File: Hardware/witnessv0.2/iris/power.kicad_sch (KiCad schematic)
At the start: 28 parts, among them Q1 SQA403EJ, Q2 SQA403EJ, U2 ME6118A33PG, U6 TPS63070

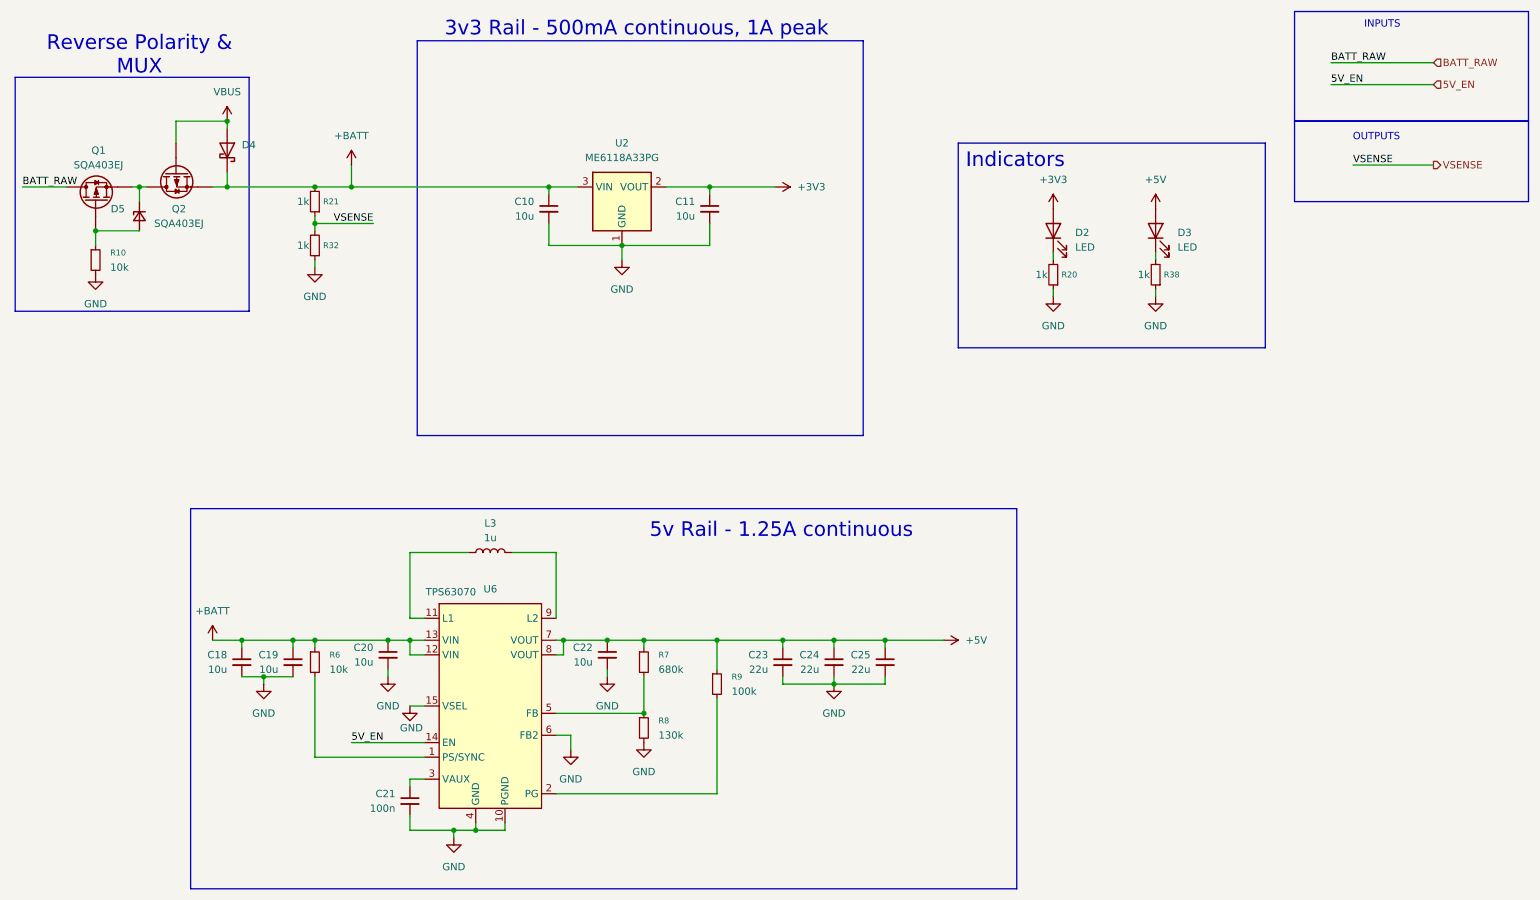
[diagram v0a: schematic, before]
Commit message: root feedback
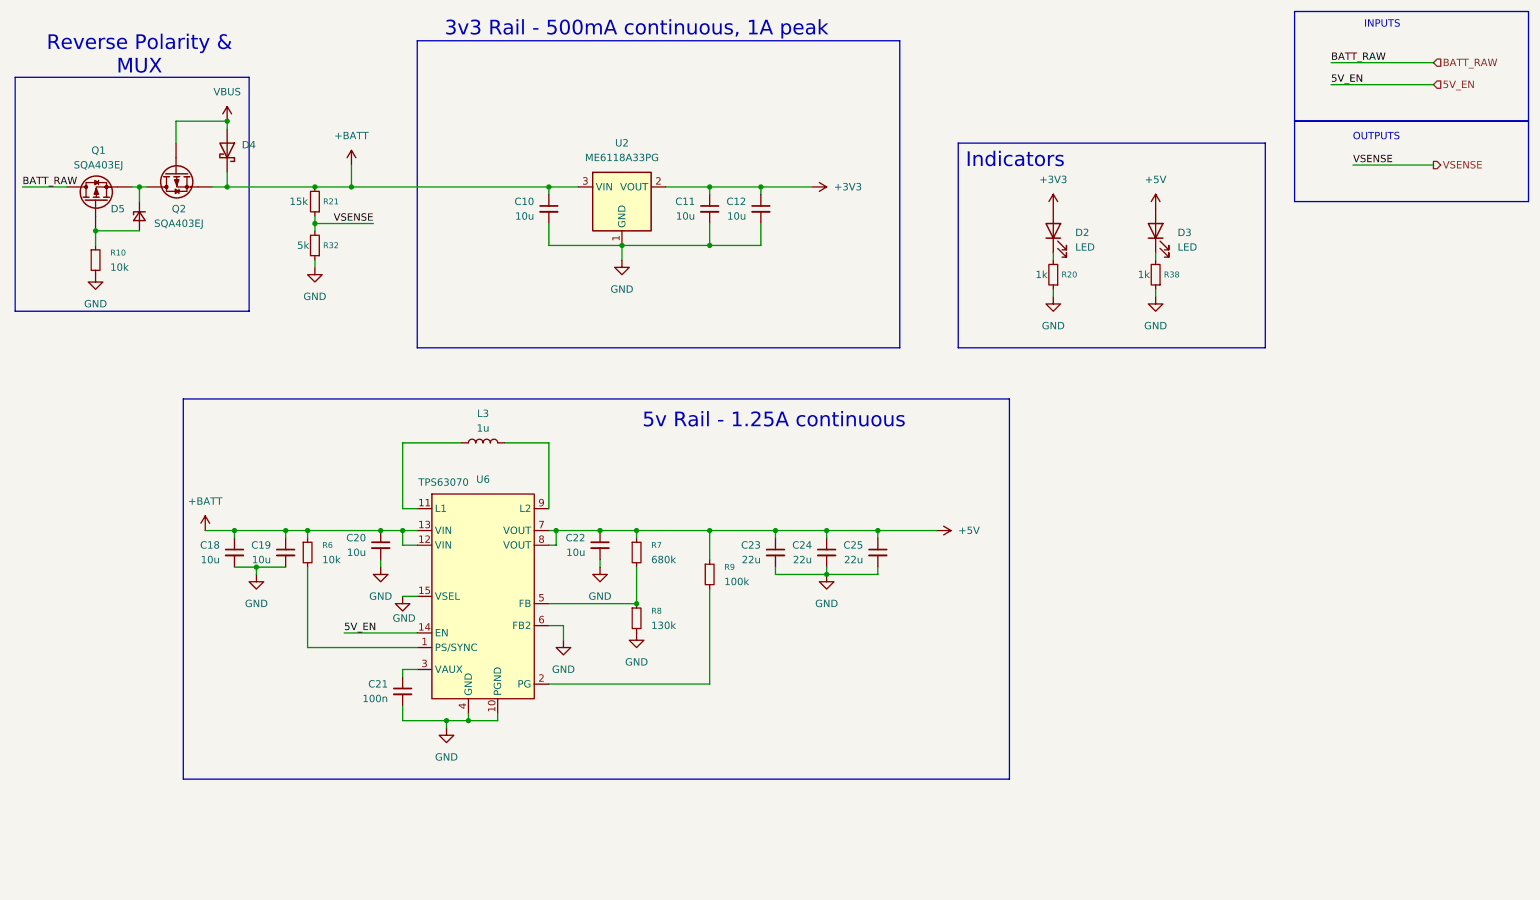
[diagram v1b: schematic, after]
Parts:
- added C12: 10u, Capacitor_SMD:C_0805_2012Metric, symbol Device:C_Small
- R21: value 1k -> 15k; LCSC_Part C11702 -> (none)
- R32: value 1k -> 5k; LCSC_Part C11702 -> (none)
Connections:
- net +3V3: now also C12.1
- net GND: now also C12.2
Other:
- moved on the sheet: C18, C19, C20, C21, C22, C23, C24, C25, L3, R6, R7, R8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
